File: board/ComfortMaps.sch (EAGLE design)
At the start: 42 parts, among them J1 PROG_HDR, J5 0545482271, J6 0545482271, U1 ADXL362, U3 ADP160-3.3, U4 MCP73833, X1 RASPI_GPIO_B+#_PIN

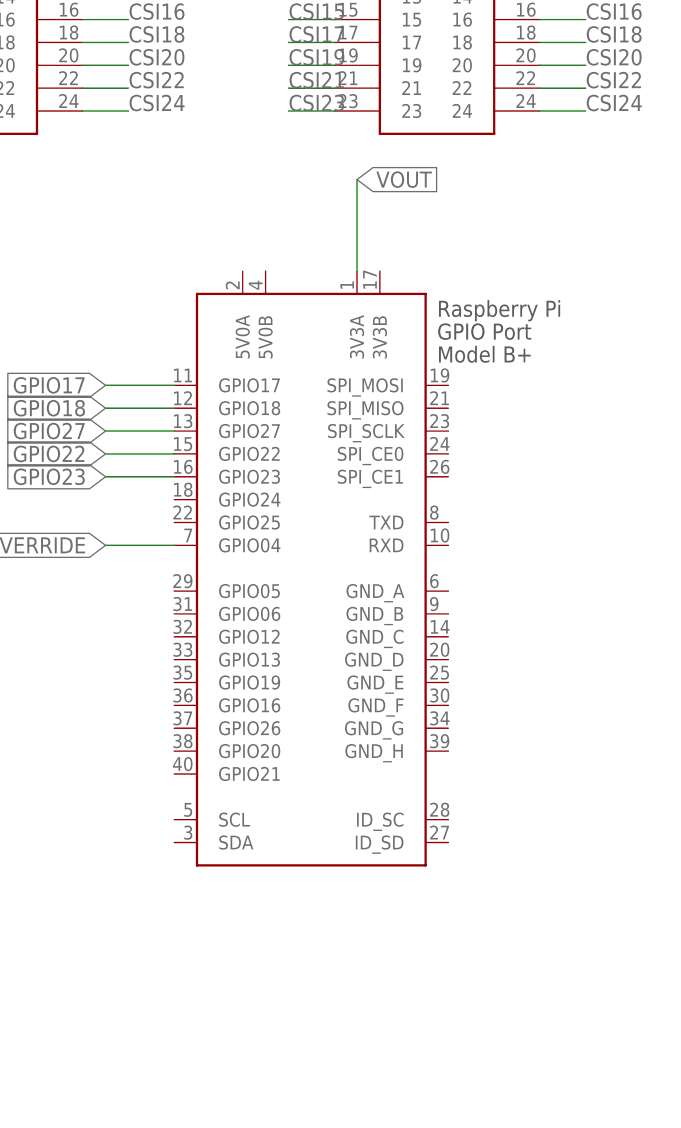
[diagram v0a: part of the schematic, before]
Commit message: Updating board, needs components on digikey.
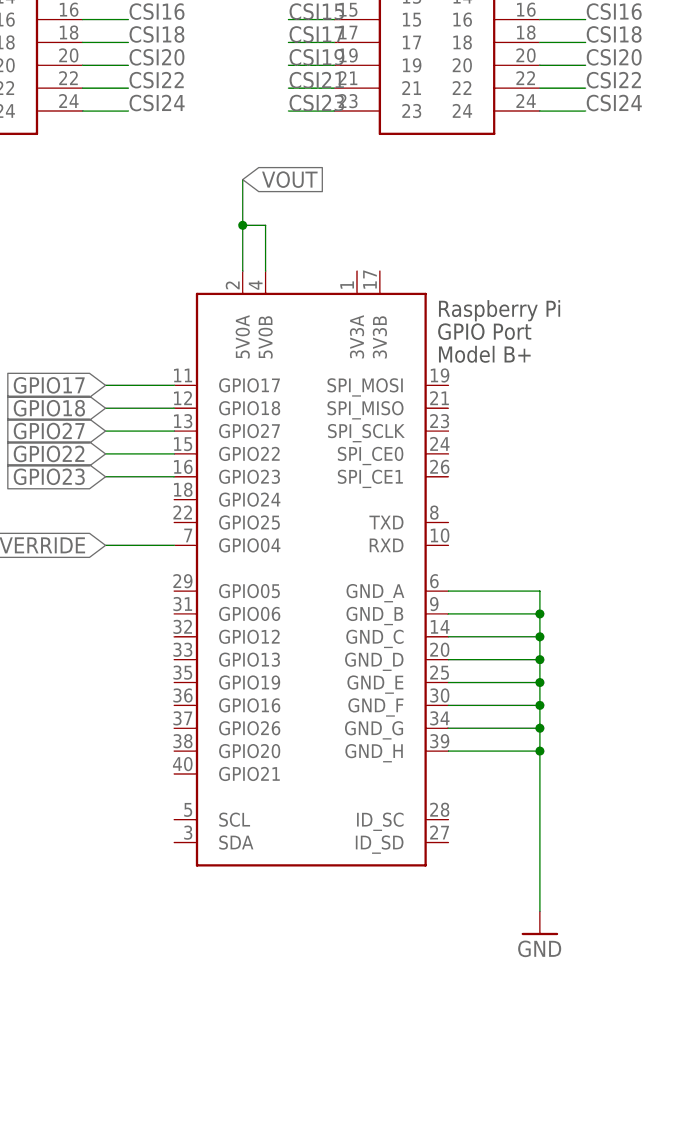
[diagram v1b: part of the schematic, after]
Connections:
- net GND: now also X1.GND_A, X1.GND_B, X1.GND_C, X1.GND_D, X1.GND_E, X1.GND_F, X1.GND_G, X1.GND_H
- net VOUT: now also X1.5V0A, X1.5V0B; no longer X1.3V3A
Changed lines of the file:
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@@
 <part name="J5" library="0545482271" deviceset="0545482271" device=""/>
 <part name="J6" library="0545482271" deviceset="0545482271" device=""/>
+<part name="GND8" library="SparkFun-Aesthetics" deviceset="GND" device=""/>
 </parts>
 <sheets>
@@
 <attribute name="NAME" x="326.39" y="147.32" size="1.778" layer="95" align="center-left"/>
 <attribute name="VALUE" x="326.39" y="144.78" size="1.778" layer="96" align="center-left"/>
+</instance>
+<instance part="GND8" gate="1" x="330.2" y="20.32" smashed="yes">
+<attribute name="VALUE" x="327.66" y="17.78" size="1.778" layer="96"/>
 </instance>
 </instances>
@@
 </segment>
 <segment>
-<pinref part="X1" gate="G$1" pin="3V3A"/>
-<wire x1="309.88" y1="93.98" x2="309.88" y2="104.14" width="0.1524" layer="91"/>
-<label x="309.88" y="104.14" size="1.778" layer="95" xref="yes"/>
+<label x="297.18" y="104.14" size="1.778" layer="95" xref="yes"/>
+<pinref part="X1" gate="G$1" pin="5V0A"/>
+<wire x1="297.18" y1="93.98" x2="297.18" y2="99.06" width="0.1524" layer="91"/>
+<pinref part="X1" gate="G$1" pin="5V0B"/>
+<wire x1="297.18" y1="99.06" x2="297.18" y2="104.14" width="0.1524" layer="91"/>
+<wire x1="299.72" y1="93.98" x2="299.72" y2="99.06" width="0.1524" layer="91"/>
+<wire x1="299.72" y1="99.06" x2="297.18" y2="99.06" width="0.1524" layer="91"/>
+<junction x="297.18" y="99.06"/>
 </segment>
 </net>
@@
 <pinref part="GND19" gate="1" pin="GND"/>
 </segment>
+<segment>
+<pinref part="X1" gate="G$1" pin="GND_A"/>
+<pinref part="GND8" gate="1" pin="GND"/>
+<wire x1="320.04" y1="58.42" x2="330.2" y2="58.42" width="0.1524" layer="91"/>
+<wire x1="330.2" y1="58.42" x2="330.2" y2="55.88" width="0.1524" layer="91"/>
+<pinref part="X1" gate="G$1" pin="GND_B"/>
+<wire x1="330.2" y1="55.88" x2="330.2" y2="53.34" width="0.1524" layer="91"/>
+<wire x1="330.2" y1="53.34" x2="330.2" y2="50.8" width="0.1524" layer="91"/>
+<wire x1="330.2" y1="50.8" x2="330.2" y2="48.26" width="0.1524" layer="91"/>
+<wire x1="330.2" y1="48.26" x2="330.2" y2="45.72" width="0.1524" layer="91"/>
+<wire x1="330.2" y1="45.72" x2="330.2" y2="43.18" width="0.1524" layer="91"/>
+<wire x1="330.2" y1="43.18" x2="330.2" y2="40.64" width="0.1524" layer="91"/>
+<wire x1="330.2" y1="40.64" x2="330.2" y2="22.86" width="0.1524" layer="91"/>
+<wire x1="320.04" y1="55.88" x2="330.2" y2="55.88" width="0.1524" layer="91"/>
+<junction x="330.2" y="55.88"/>
+<pinref part="X1" gate="G$1" pin="GND_C"/>
+<wire x1="320.04" y1="53.34" x2="330.2" y2="53.34" width="0.1524" layer="91"/>
+<junction x="330.2" y="53.34"/>
+<pinref part="X1" gate="G$1" pin="GND_D"/>
+<wire x1="320.04" y1="50.8" x2="330.2" y2="50.8" width="0.1524" layer="91"/>
+<junction x="330.2" y="50.8"/>
+<pinref part="X1" gate="G$1" pin="GND_E"/>
+<wire x1="320.04" y1="48.26" x2="330.2" y2="48.26" width="0.1524" layer="91"/>
+<junction x="330.2" y="48.26"/>
+<pinref part="X1" gate="G$1" pin="GND_F"/>
+<wire x1="320.04" y1="45.72" x2="330.2" y2="45.72" width="0.1524" layer="91"/>
+<junction x="330.2" y="45.72"/>
+<pinref part="X1" gate="G$1" pin="GND_G"/>
+<wire x1="320.04" y1="43.18" x2="330.2" y2="43.18" width="0.1524" layer="91"/>
+<junction x="330.2" y="43.18"/>
+<pinref part="X1" gate="G$1" pin="GND_H"/>
+<wire x1="320.04" y1="40.64" x2="330.2" y2="40.64" width="0.1524" layer="91"/>
+<junction x="330.2" y="40.64"/>
+</segment>
 </net>

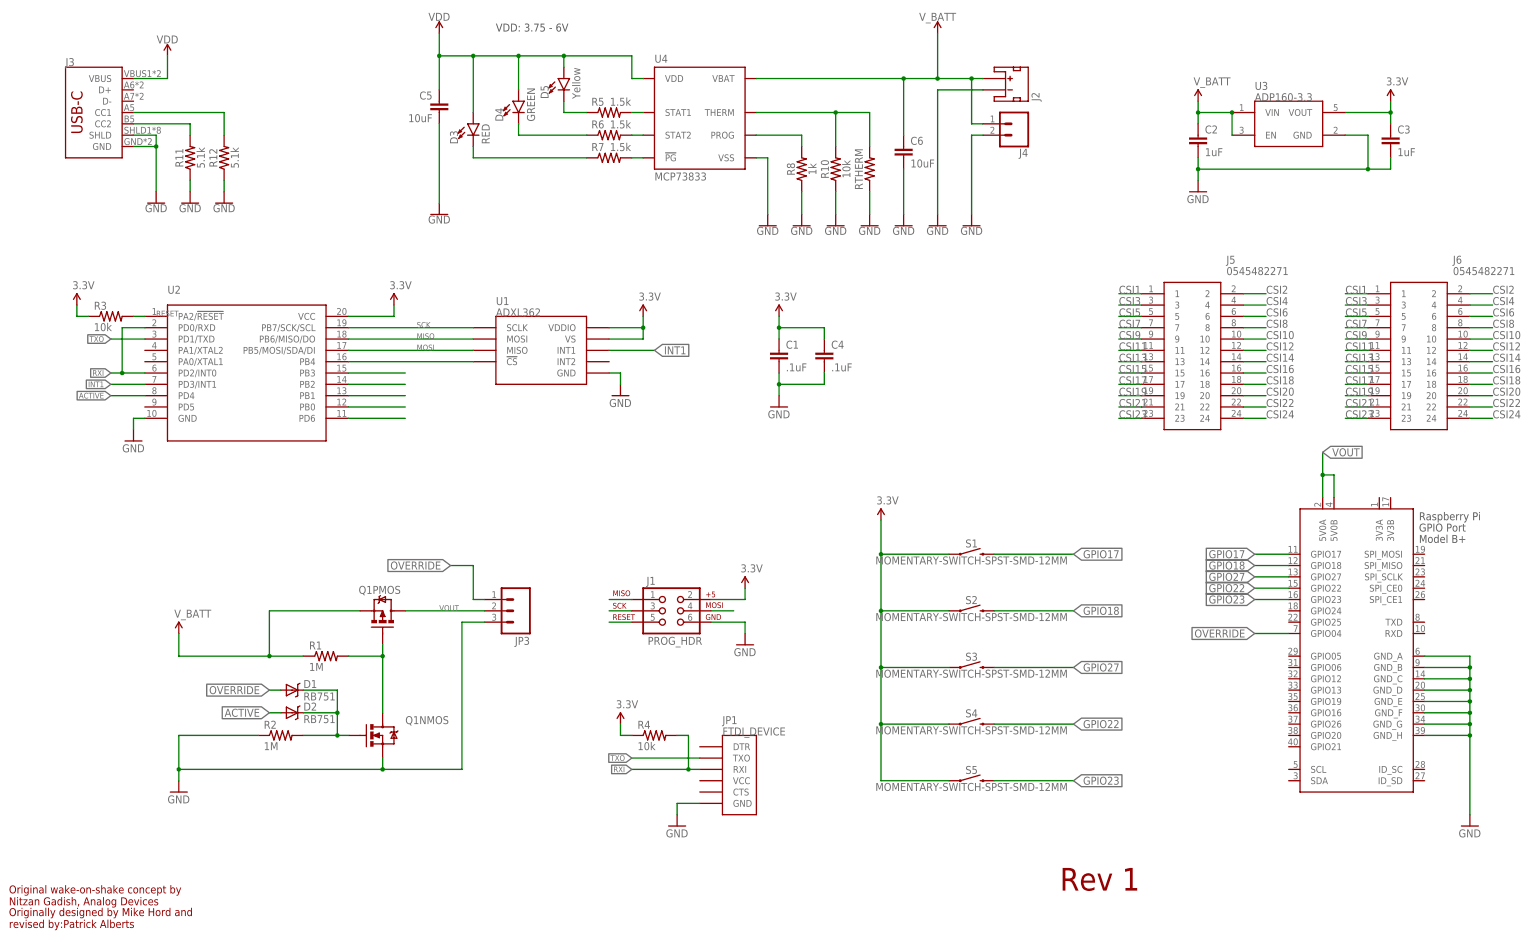
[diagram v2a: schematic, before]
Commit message: Soldering first board.
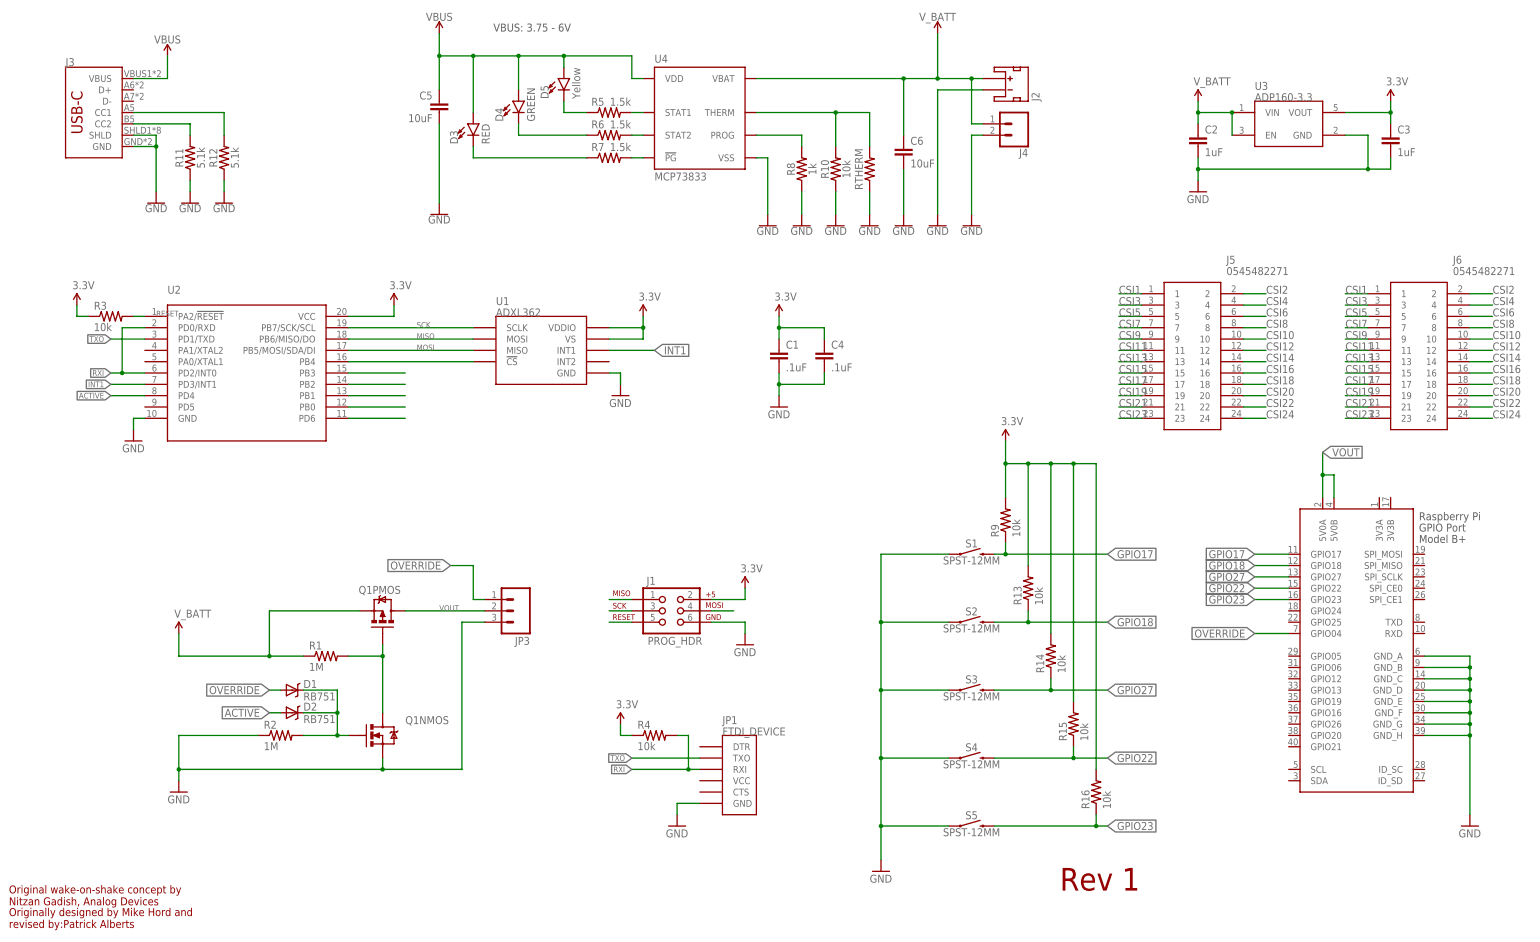
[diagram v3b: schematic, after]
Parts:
- added R13, R14, R15, R16, R9: 10k, SparkFun-Resistors:10K-1%RES-00824
- S1, S2, S3, S4, S5: value MOMENTARY-SWITCH-SPST-SMD-12MM -> SPST-12MM
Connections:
- net VDD renamed V_USB
- net 3.3V: now also R13.2, R14.2, R15.2, R16.2, R9.2; no longer S1.1, S2.1, S3.1, S4.1, S5.1
- net GND: now also S1.1, S2.1, S3.1, S4.1, S5.1
- net GPIO17: now also R9.1
- net GPIO18: now also R13.1
- net GPIO22: now also R15.1
- net GPIO23: now also R16.1
- net GPIO27: now also R14.1
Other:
- note added: "VBUS: 3.75 - 6V"
- note removed: "VDD: 3.75 - 6V"
- moved on the sheet: S2, S3, S4, S5
